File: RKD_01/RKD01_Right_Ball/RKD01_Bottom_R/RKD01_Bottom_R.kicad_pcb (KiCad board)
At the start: 2 copper layers, 202.4 x 126.2 mm, 8 parts, among them M1 Mark, M2 Mark, M3 Mark, M4 Mark, M5 Mark, M6 Mark, M7 Mark, M8 Mark

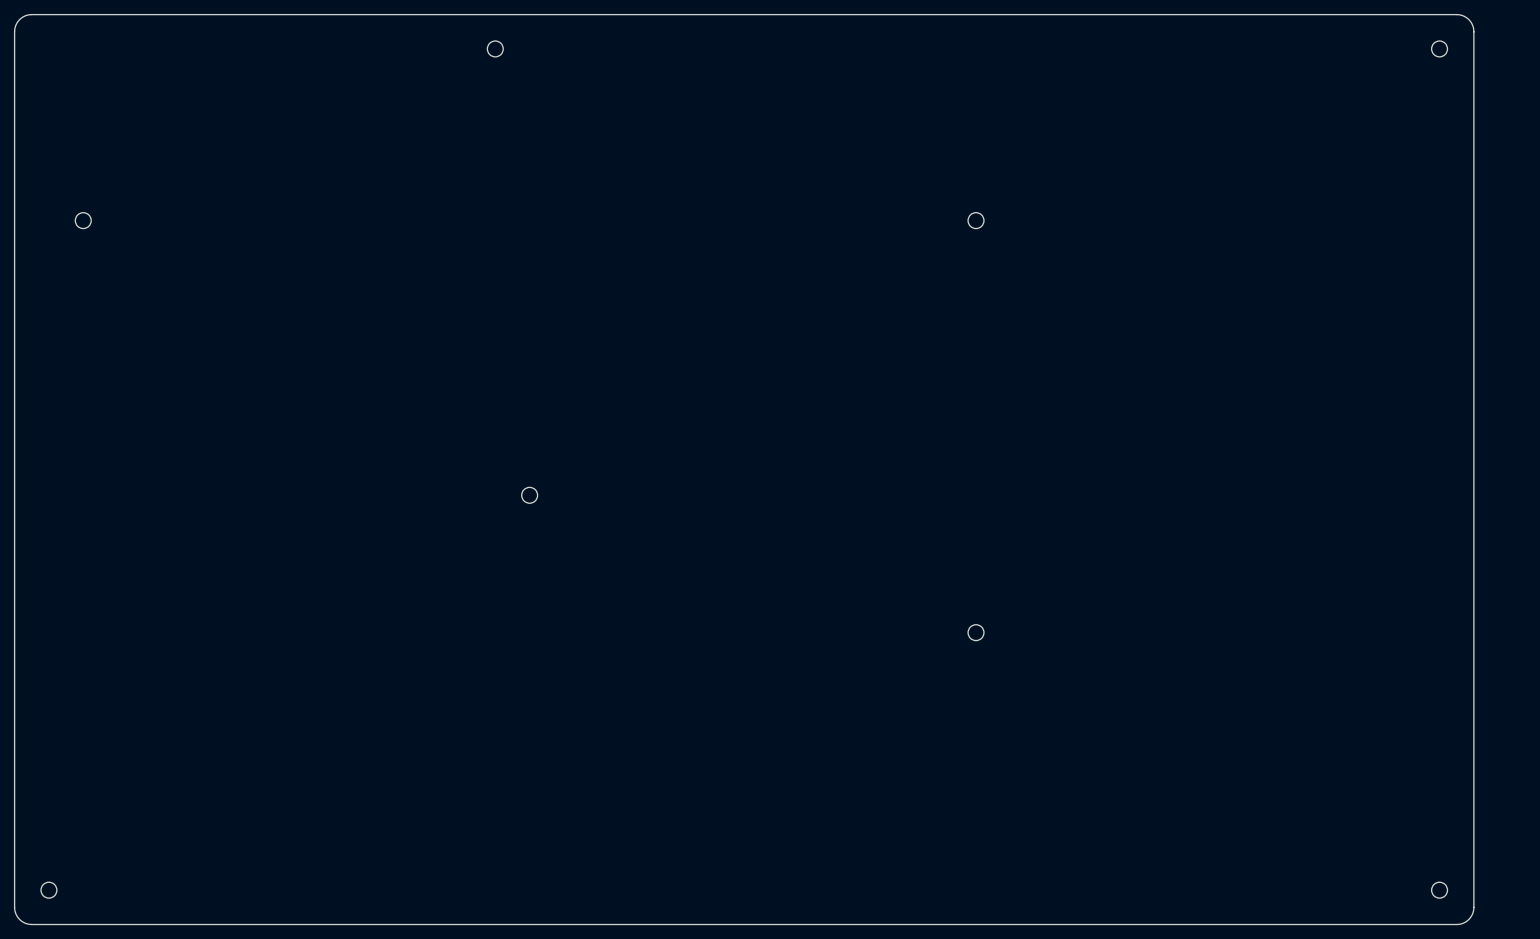
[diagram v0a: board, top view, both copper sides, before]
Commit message: デザイン見直し
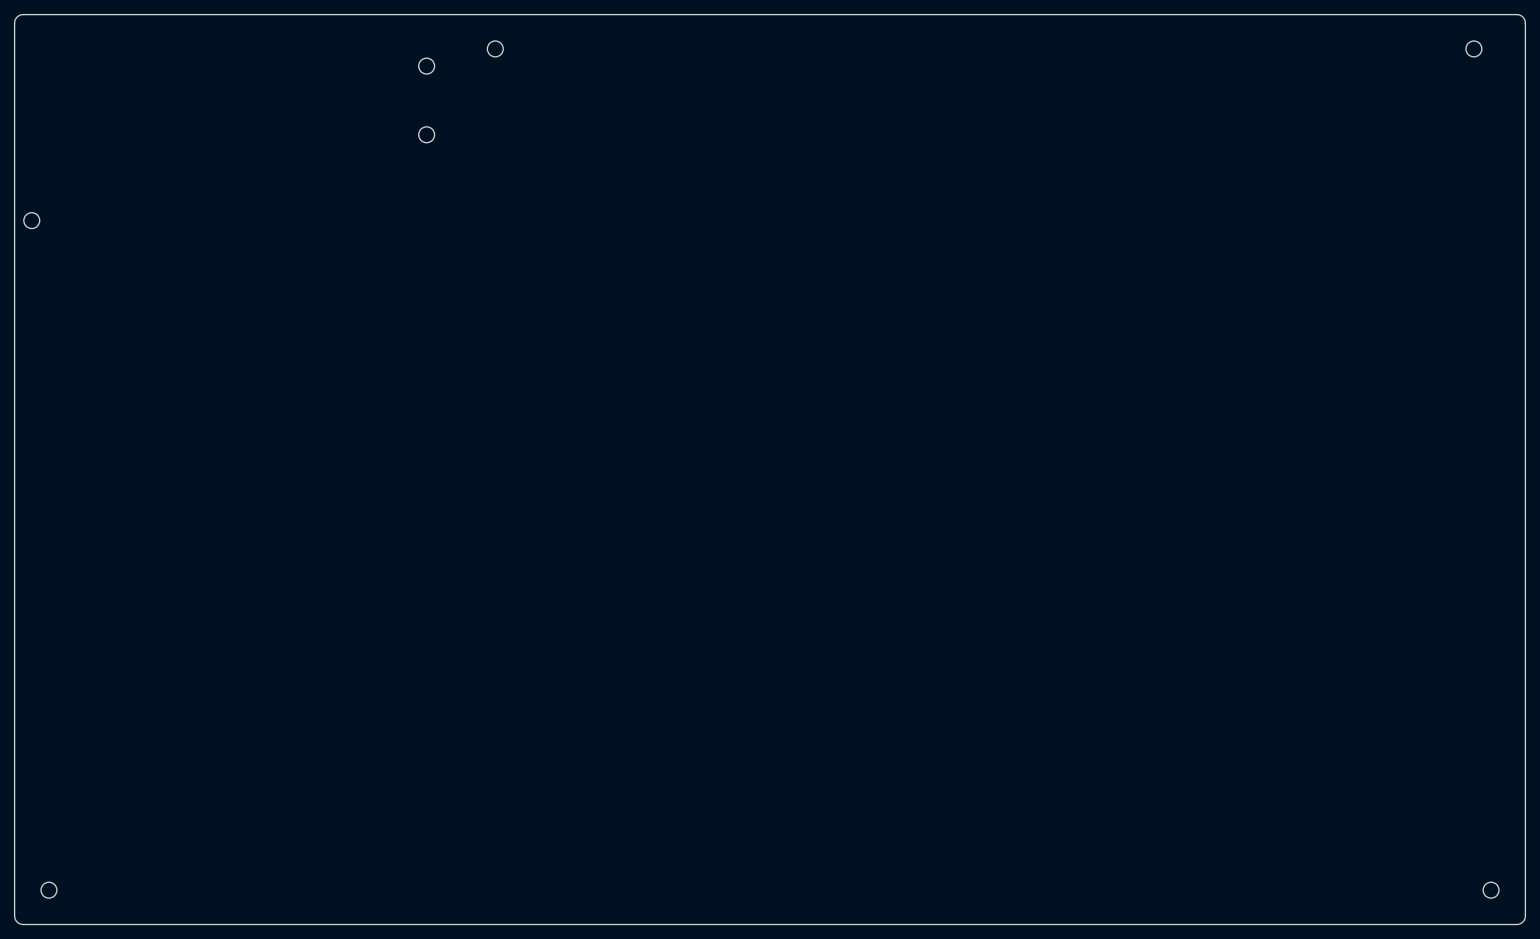
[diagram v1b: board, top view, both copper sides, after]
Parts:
- removed M8: Mark, kbd_Hole:m2_Screw_Hole
- moved M4 117.2 mm to (226.2, 140.5)
- moved M6 102.8 mm to (78.6, 35.7)
- moved M3 93.0 mm to (26.2, 140.5)
- moved M7 92.9 mm to (23.8, 47.6)
- moved M5 61.2 mm to (78.6, 26.2)
- moved M2 4.76 mm to (223.8, 23.8)
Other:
- board size 202.4 x 126.2 mm -> 209.5 x 126.2 mm
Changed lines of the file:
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@@
 	(footprint "kbd_Hole:m2_Screw_Hole"
 		(layer "F.Cu")
-		(at 219.075 23.8125)
+		(at 223.8375 23.8125)
 		(descr "Mounting Hole 2.2mm, no annular, M2")
 		(tags "mounting hole 2.2mm no annular m2")
@@
 	(footprint "kbd_Hole:m2_Screw_Hole"
 		(layer "F.Cu")
-		(at 92.8688 85.725)
+		(at 23.8125 47.625)
 		(descr "Mounting Hole 2.2mm, no annular, M2")
 		(tags "mounting hole 2.2mm no annular m2")
-		(property "Reference" "M5"
+		(property "Reference" "M7"
 			(at 0 -3.2 0)
 			(layer "F.Fab")
@@
 			)
 		)
-		(sheetname "ルート")
-		(sheetfile "RKD01_Assemble_R.kicad_sch")
-		(attr exclude_from_pos_files exclude_from_bom)
+		(attr exclude_from_pos_files)
 		(fp_circle
 			(center 0 0)
@@
 	(footprint "kbd_Hole:m2_Screw_Hole"
 		(layer "F.Cu")
-		(at 26.19375 140.49375)
+		(at 78.5813 26.1937)
 		(descr "Mounting Hole 2.2mm, no annular, M2")
 		(tags "mounting hole 2.2mm no annular m2")
-		(property "Reference" "M7"
+		(property "Reference" "M5"
 			(at 0 -3.2 0)
 			(layer "F.Fab")
@@
 		(sheetname "ルート")
 		(sheetfile "RKD01_Assemble_R.kicad_sch")
-		(attr exclude_from_pos_files exclude_from_bom)
+		(attr exclude_from_pos_files)
 		(fp_circle
 			(center 0 0)
@@
 	(footprint "kbd_Hole:m2_Screw_Hole"
 		(layer "F.Cu")
-		(at 219.075 140.4937)
+		(at 226.21875 140.4937)
 		(descr "Mounting Hole 2.2mm, no annular, M2")
 		(tags "mounting hole 2.2mm no annular m2")
-		(property "Reference" "M8"
+		(property "Reference" "M4"
 			(at 0 -3.2 0)
 			(layer "F.Fab")
@@
 	(footprint "kbd_Hole:m2_Screw_Hole"
 		(layer "F.Cu")
-		(at 154.7813 47.625)
+		(at 78.5813 35.7187)
 		(descr "Mounting Hole 2.2mm, no annular, M2")
 		(tags "mounting hole 2.2mm no annular m2")
-		(property "Reference" "M4"
+		(property "Reference" "M6"
 			(at 0 -3.2 0)
 			(layer "F.Fab")
@@
 		(sheetname "ルート")
 		(sheetfile "RKD01_Assemble_R.kicad_sch")
-		(attr exclude_from_pos_files exclude_from_bom)
+		(attr exclude_from_pos_files)
 		(fp_circle
 			(center 0 0)
@@
 	(footprint "kbd_Hole:m2_Screw_Hole"
 		(layer "F.Cu")
-		(at 88.10625 23.8125)
+		(at 88.1063 23.8125)
 		(descr "Mounting Hole 2.2mm, no annular, M2")
 		(tags "mounting hole 2.2mm no annular m2")
@@
 	(footprint "kbd_Hole:m2_Screw_Hole"
 		(layer "F.Cu")
-		(at 30.9563 47.625)
+		(at 26.1938 140.4937)
 		(descr "Mounting Hole 2.2mm, no annular, M2")
 		(tags "mounting hole 2.2mm no annular m2")
@@
 		)
 	)
-	(footprint "kbd_Hole:m2_Screw_Hole"
-		(layer "F.Cu")
-		(at 154.7813 104.775)
-		(descr "Mounting Hole 2.2mm, no annular, M2")
-		(tags "mounting hole 2.2mm no annular m2")
-		(property "Reference" "M6"
-			(at 0 -3.2 0)
-			(layer "F.Fab")
-			(effects
-				(font
-					(size 1 1)
-					(thickness 0.15)
-				)
-			)
-		)
-		(property "Value" "Mark"
-			(at 0 3.2 0)
-			(layer "F.Fab")
-			(effects
-				(font
-					(size 1 1)
-					(thickness 0.15)
-				)
-			)
-		)
-		(property "Footprint" "kbd_Hole:m2_Screw_Hole"
-			(at 0 0 0)
-			(layer "F.Fab")
-			(hide yes)
-			(effects
-				(font
-					(size 1.27 1.27)
-					(thickness 0.15)
-				)
-			)
-		)
-		(property "Datasheet" ""
-			(at 0 0 0)
-			(layer "F.Fab")
-			(hide yes)
-			(effects
-				(font
-					(size 1.27 1.27)
-					(thickness 0.15)
-				)
-			)
-		)
-		(property "Description" ""
-			(at 0 0 0)
-			(layer "F.Fab")
-			(hide yes)
-			(effects
-				(font
-					(size 1.27 1.27)
-					(thickness 0.15)
-				)
-			)
-		)
-		(attr exclude_from_pos_files exclude_from_bom)
-		(fp_circle
-			(center 0 0)
-			(end 2.2 0)
-			(stroke
-				(width 0.15)
-				(type solid)
-			)
-			(fill none)
-			(layer "Cmts.User")
-		)
-		(fp_circle
-			(center 0 0)
-			(end 2.45 0)
-			(stroke
-				(width 0.05)
-				(type solid)
-			)
-			(fill none)
-			(layer "F.CrtYd")
-		)
-		(fp_text user "${REFERENCE}"
-			(at 0.3 0 0)
-			(layer "F.Fab")
-			(effects
-				(font
-					(size 1 1)
-					(thickness 0.15)
-				)
-			)
-		)
-		(pad "" np_thru_hole circle
-			(at 0 0)
-			(size 2.2 2.2)
-			(drill 2.2)
-			(layers "*.Cu" "*.Mask")
-		)
-	)
 	(gr_line
-		(start 221.4563 145.25625)
-		(end 23.8125 145.25625)
+		(start 229.790625 145.25625)
+		(end 22.621875 145.25625)
 		(stroke
 			(width 0.05)
@@
 		(layer "Edge.Cuts")
 	)
-	(gr_arc
-		(start 21.43125 21.43125)
-		(mid 22.128702 19.747452)
-		(end 23.8125 19.05)
+	(gr_line
+		(start 21.43125 144.065625)
+		(end 21.4313 20.240625)
 		(stroke
 			(width 0.05)
@@
 		(layer "Edge.Cuts")
 	)
-	(gr_arc
-		(start 23.8125 145.25625)
-		(mid 22.128702 144.558798)
-		(end 21.43125 142.875)
+	(gr_line
+		(start 230.98125 20.240625)
+		(end 230.98125 144.065625)
 		(stroke
 			(width 0.05)
@@
 		(layer "Edge.Cuts")
 	)
-	(gr_line
-		(start 21.43125 142.875)
-		(end 21.43125 21.43125)
+	(gr_arc
+		(start 229.790625 19.05)
+		(mid 230.632524 19.398726)
+		(end 230.98125 20.240625)
 		(stroke
 			(width 0.05)
@@
 	)
 	(gr_line
-		(start 223.8375 21.43125)
-		(end 223.8375 142.875)
+		(start 229.790625 19.05)
+		(end 22.621875 19.05005)
 		(stroke
 			(width 0.05)
@@
 		(layer "Edge.Cuts")
 	)
-	(gr_line
-		(start 221.4562 19.05)
-		(end 23.8125 19.05)
+	(gr_arc
+		(start 21.4313 20.240625)
+		(mid 21.780011 19.398761)
+		(end 22.621875 19.05005)
 		(stroke
 			(width 0.05)
@@
 	)
 	(gr_arc
-		(start 223.83755 142.875)
-		(mid 223.140101 144.558816)
-		(end 221.4563 145.25625)
+		(start 230.98125 144.065625)
+		(mid 230.632524 144.907524)
+		(end 229.790625 145.25625)
 		(stroke
 			(width 0.05)
@@
 	)
 	(gr_arc
-		(start 221.4562 19.05)
-		(mid 223.140013 19.747437)
-		(end 223.83745 21.43125)
+		(start 22.621875 145.25625)
+		(mid 21.779976 144.907524)
+		(end 21.43125 144.065625)
 		(stroke
 			(width 0.05)
@@
 	)
 	(gr_text "RKD01_Right v1.0"
-		(at 209.55 23.8125 0)
+		(at 214.3125 23.8125 0)
 		(layer "B.SilkS")
 		(effects
